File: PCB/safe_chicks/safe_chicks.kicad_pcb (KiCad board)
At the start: 2 copper layers, 78 x 68 mm, 35 parts, among them J1 Conn_01x15, J10 Status LEDs, J11 UART, J12 SPI, J13 Conn_01x02, J2 Conn_01x15, J3 Battery Sensor, J4 Light Sensor, J5 Upper Switch, J6 Bottom Switch, J7 Motor, J8 5V (from PM), J9 LowPower

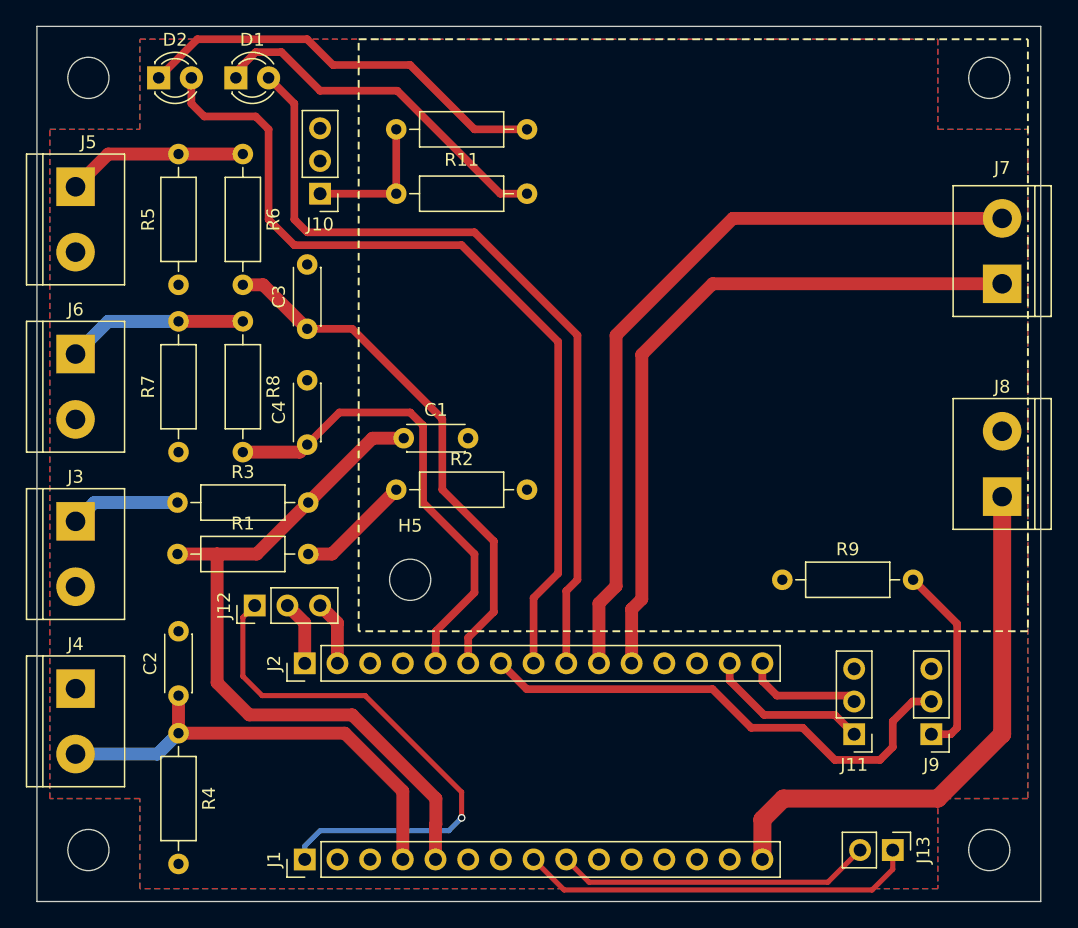
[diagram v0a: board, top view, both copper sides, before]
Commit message: Created PCB
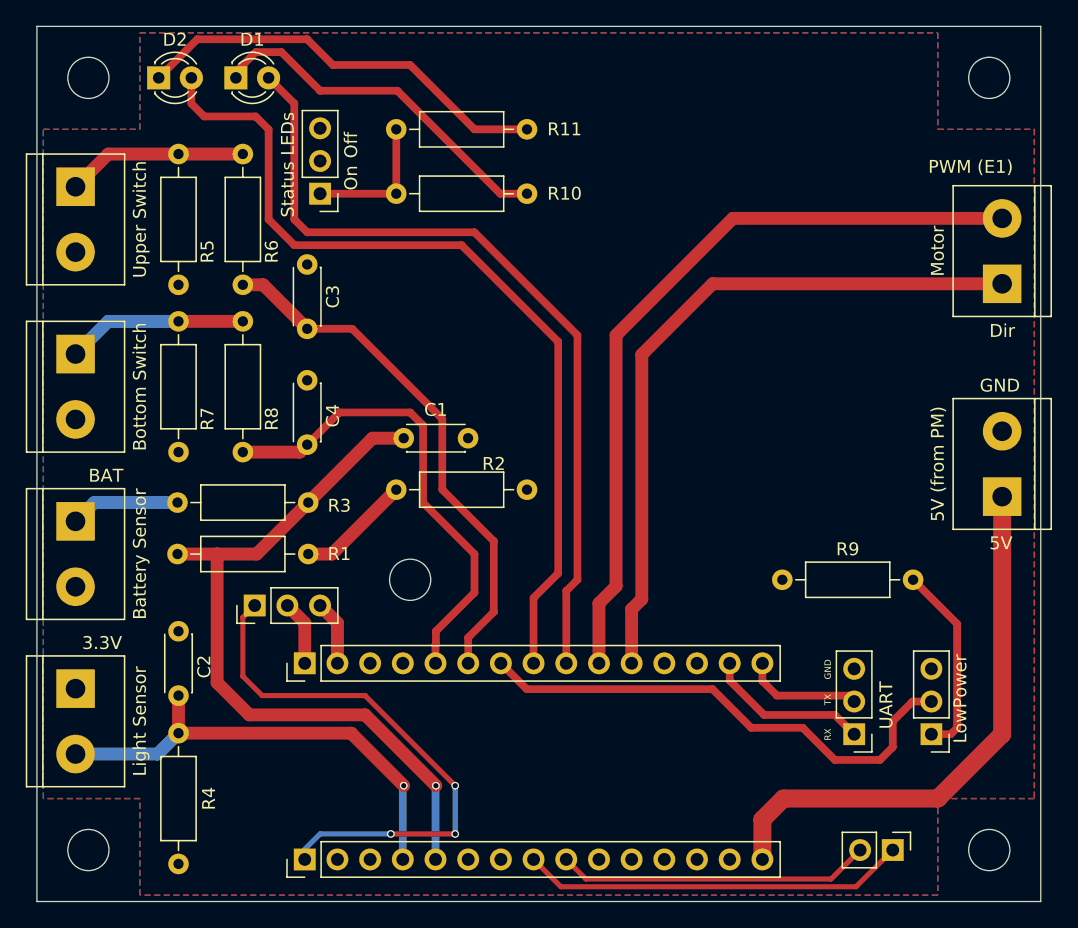
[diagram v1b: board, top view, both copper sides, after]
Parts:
- added G***: LOGO, LOGO, B.Cu at (133.0, 57.8)
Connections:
- J1 pad 13: /~{RESET} -> unconnected-(J1-Pin_13-Pad13)
- J2 pad 13: /~{RESET} -> unconnected-(J2-Pin_13-Pad13)
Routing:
- net /A4/SDA: track 31.1 -> 30.0 mm
- net /A1: track 56.8 -> 57.4 mm, vias 0 -> 1
- net /A0: track 36.2 -> 36.5 mm, vias 0 -> 1
- net /D13/SCK: track 42.7 -> 42.6 mm, vias 1 -> 3
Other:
- board text added: "3.3V"
- board text added: "5V"
- board text added: "BAT"
- board text added: "Dir"
- board text added: "GND"
- board text added: "Off"
- board text added: "On"
- board text added: "PWM (E1)"
- board text added: "RX"
- board text added: "TX"
